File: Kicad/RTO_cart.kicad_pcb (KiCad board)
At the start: 2 copper layers, 68.1 x 90.1 mm, 22 parts, among them J1 2x22 card edge connector, J2 Oled 0.91" female, SW1 SW_Push, SW2 SW_Push, SW3 SW_Push, U1 74LVC245, U2 74LVC245, U3 74LVC245, U4 Teensy4.1, U5 74LVC245

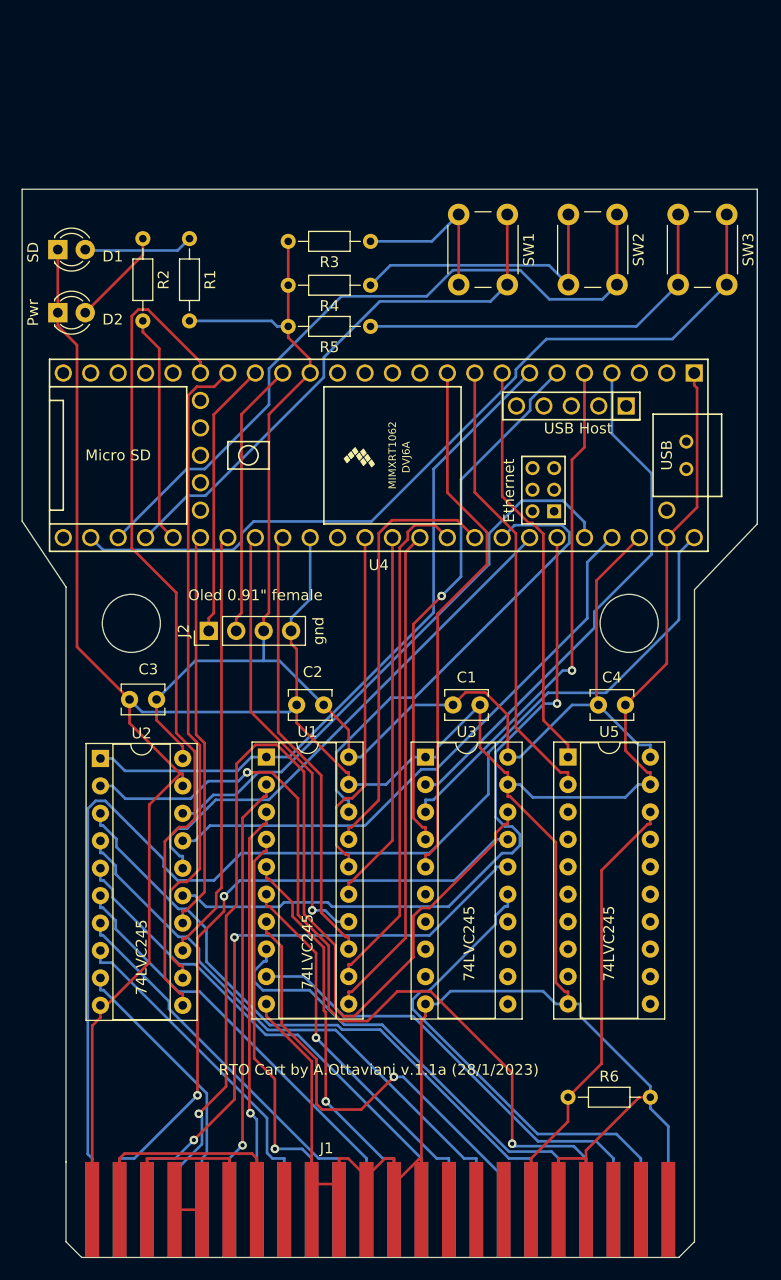
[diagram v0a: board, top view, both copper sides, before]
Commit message: Add files via upload
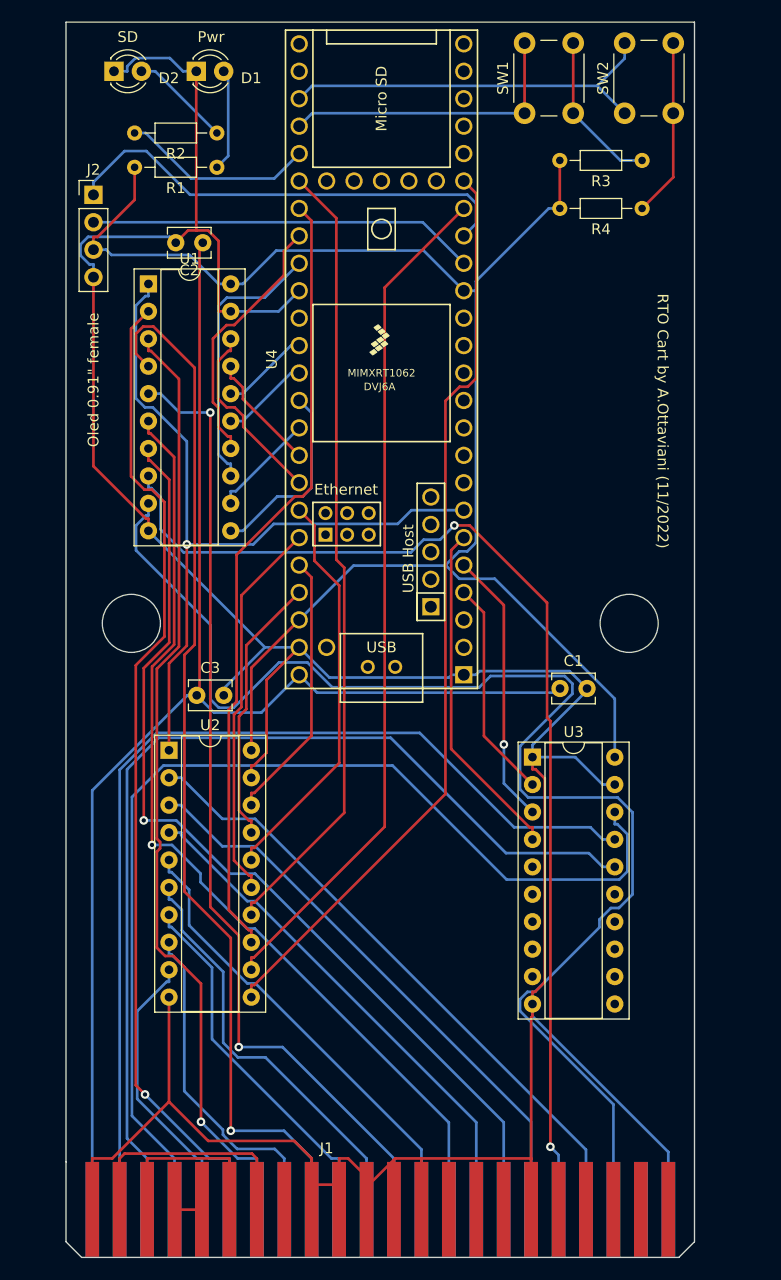
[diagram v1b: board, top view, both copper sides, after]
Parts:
- removed C4: 100nF, Capacitor_THT:C_Disc_D3.8mm_W2.6mm_P2.50mm
- removed R5: 1K, Resistor_THT:R_Axial_DIN0204_L3.6mm_D1.6mm_P7.62mm_Horizontal
- removed R6: 4K7, Resistor_THT:R_Axial_DIN0204_L3.6mm_D1.6mm_P7.62mm_Horizontal
- removed SW3: SW_Push, Button_Switch_THT:SW_PUSH_6mm
- removed U5: 74LVC245, Package_DIP:DIP-20_W7.62mm_Socket
- U1, U2, U3: value 74LVC245 -> 74LS245
- moved U1 45.2 mm to (96.5, 102.2)
- moved C2 44.2 mm to (101.6, 98.4)
- moved J2 41.8 mm to (91.4, 94.0), turned to 0 degrees
- moved R3 26.2 mm to (142.2, 90.8)
- moved R4 26.1 mm to (142.2, 95.2)
- moved D2 22.9 mm to (93.3, 82.5)
- moved D1 20.9 mm to (101.0, 82.5)
- moved R2 11.9 mm to (102.9, 88.3), turned to 180 degrees
- moved C1 10.0 mm to (134.6, 139.7)
- moved U3 9.91 mm to (132.1, 146.1)
- moved SW1 9.51 mm to (131.4, 86.4), turned to 90 degrees
- moved SW2 9.40 mm to (140.6, 86.4), turned to 90 degrees
- moved U4 8.89 mm to (118.1, 109.2), turned to 90 degrees
- moved R1 7.08 mm to (102.9, 91.4), turned to 180 degrees
- moved U2 6.40 mm to (98.4, 145.4)
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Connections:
- C1 pad 1: +3.3V -> +5V
- C2 pad 1: +3.3V -> +5V
- C3 pad 1: +3.3V -> +5V
- J1 pad 10: GND -> unconnected-(J1-Pad10)
- J1 pad 12: rst' -> GND
- J1 pad 3: ~{msync'} -> unconnected-(J1-Pad3)
- J1 pad 8: GND -> unconnected-(J1-Pad8)
- U3 pad 15: ~{msync'} -> unconnected-(U3-Pad15)
- U3 pad 5: ~{MSYNC} -> unconnected-(U3-Pad5)
- U4 pad 10: ~{MSYNC} -> unconnected-(U4-Pad10)
- U4 pad 26: BT3 -> unconnected-(U4-Pad26)
- U4 pad 8: DIR2 -> unconnected-(U4-Pad8)
- U4 pad 9: RST -> unconnected-(U4-Pad9)
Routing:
- net d7': track 43.9 -> 127.5 mm
- net BT3: track 76.9 -> 0.00 mm
- net d6': track 43.3 -> 102.9 mm, vias 0 -> 2
- net d2': track 38.6 -> 96.9 mm
- net d3': track 37.4 -> 89.7 mm, vias 1 -> 2
- net GND: track 368.8 -> 317.9 mm
- net d4': track 37.0 -> 87.9 mm
- net d1': track 37.9 -> 88.4 mm
- net d0': track 40.9 -> 91.3 mm
- net ~{MSYNC}: track 49.8 -> 0.00 mm
- net ~{msync'}: track 46.5 -> 0.00 mm
- net d5': track 44.6 -> 89.3 mm
- net RST: track 42.1 -> 0.00 mm
- net rst': track 41.5 -> 0.00 mm
- net DIR2: track 38.3 -> 0.00 mm
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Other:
- board size 68.1 x 90.1 mm -> 58.2 x 105.5 mm
- board text added: "RTO Cart by A.Ottaviani (11/2022)"
- board text removed: "RTO Cart by A.Ottaviani v.1.1a (28/1/2023)"
- board text removed: "gnd"

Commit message: Add files via upload
corrected the level shifter ICs to 74LVC245 instead of wrong typed 74LS245: WARNING! use only 74LVC245 chips, the other types could damage your Teensy becouse they output 5V instead of 3V3!
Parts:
- U1, U2, U3: value 74LS245 -> 74LVC245
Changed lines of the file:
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@@
       (effects (font (size 1 1) (thickness 0.15)))
     )
-    (fp_text value "74LS245" (at 3.81 25.19) (layer "F.Fab")
+    (fp_text value "74LVC245" (at 3.81 25.19) (layer "F.Fab")
       (effects (font (size 1 1) (thickness 0.15)))
     )
@@
       (effects (font (size 1 1) (thickness 0.15)))
     )
-    (fp_text value "74LS245" (at 3.81 25.19) (layer "F.Fab")
+    (fp_text value "74LVC245" (at 3.81 25.19) (layer "F.Fab")
       (effects (font (size 1 1) (thickness 0.15)))
     )
@@
       (effects (font (size 1 1) (thickness 0.15)))
     )
-    (fp_text value "74LS245" (at 3.81 25.19) (layer "F.Fab")
+    (fp_text value "74LVC245" (at 3.81 25.19) (layer "F.Fab")
       (effects (font (size 1 1) (thickness 0.15)))
     )

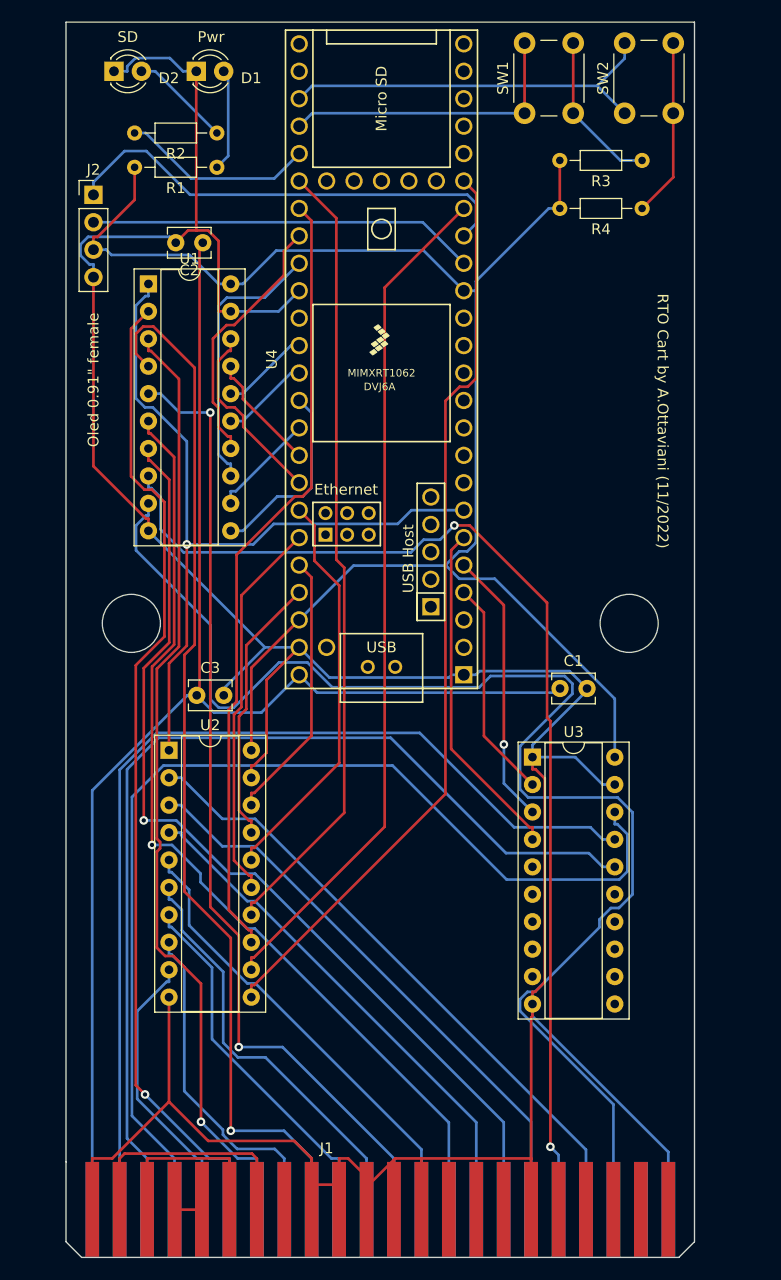
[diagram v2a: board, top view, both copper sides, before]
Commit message: Add files via upload
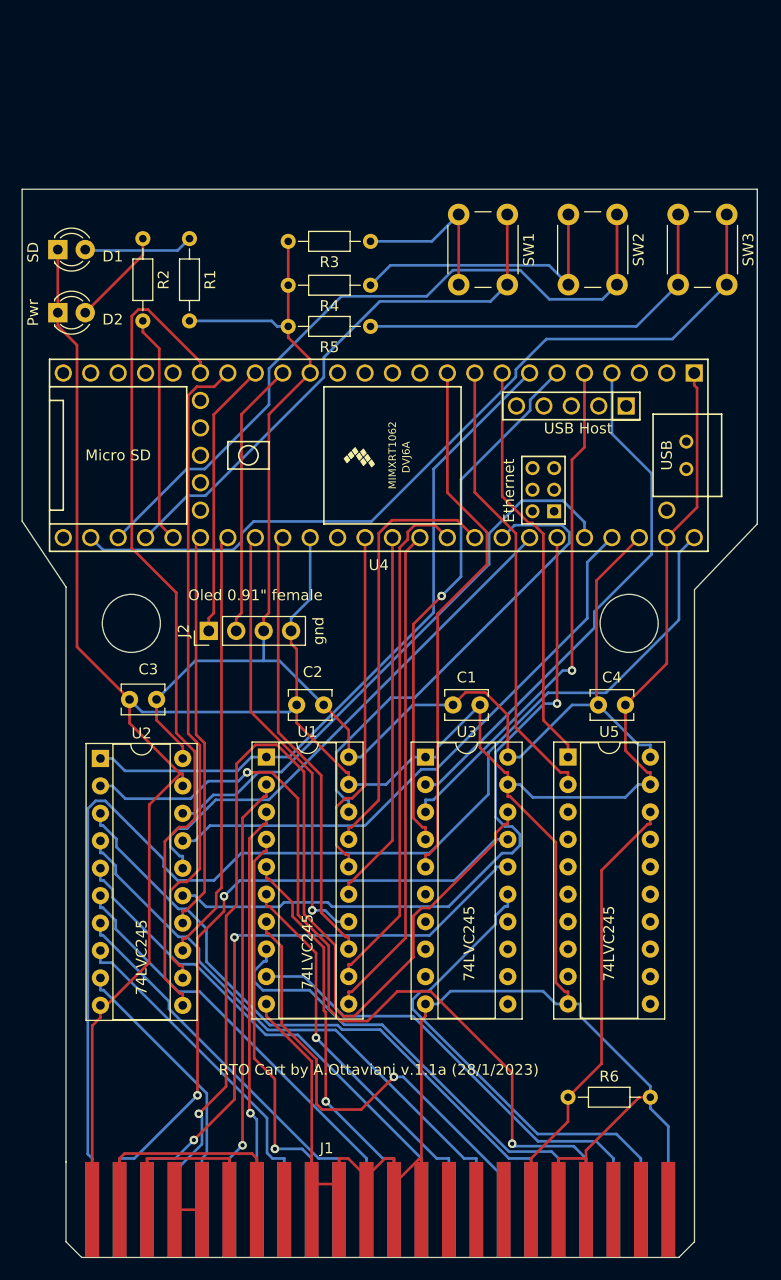
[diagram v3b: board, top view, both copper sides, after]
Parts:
- added C4: 100nF, Capacitor_THT:C_Disc_D3.8mm_W2.6mm_P2.50mm, F.Cu at (138.2, 141.2)
- added R5: 1K, Resistor_THT:R_Axial_DIN0204_L3.6mm_D1.6mm_P7.62mm_Horizontal, F.Cu at (117.1, 106.2)
- added R6: 4K7, Resistor_THT:R_Axial_DIN0204_L3.6mm_D1.6mm_P7.62mm_Horizontal, F.Cu at (135.4, 177.5)
- added SW3: SW_Push, Button_Switch_THT:SW_PUSH_6mm, F.Cu at (150.1, 95.8)
- added U5: 74LVC245, Package_DIP:DIP-20_W7.62mm_Socket, F.Cu at (135.4, 146.1)
- moved U1 45.2 mm to (107.5, 146.1)
- moved C2 44.2 mm to (112.8, 141.2)
- moved J2 41.8 mm to (102.1, 134.4), turned to 90 degrees
- moved R3 26.2 mm to (117.1, 98.3)
- moved R4 26.1 mm to (117.1, 102.4)
- moved D2 22.9 mm to (88.1, 104.9)
- moved D1 20.9 mm to (88.1, 99.1)
- moved R2 11.9 mm to (96.0, 98.0), turned to -90 degrees
- moved C1 10.0 mm to (124.7, 141.2)
- moved U3 9.91 mm to (122.2, 146.1)
- moved SW1 9.51 mm to (129.8, 95.8), turned to -90 degrees
- moved SW2 9.40 mm to (139.9, 95.8), turned to -90 degrees
- moved U4 8.89 mm to (117.9, 118.1), turned to 180 degrees
- moved R1 7.08 mm to (100.3, 98.0), turned to -90 degrees
- moved U2 6.40 mm to (92.1, 146.2)
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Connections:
- C1 pad 1: +5V -> +3.3V
- C2 pad 1: +5V -> +3.3V
- C3 pad 1: +5V -> +3.3V
- J1 pad 10: unconnected-(J1-Pad10) -> GND
- J1 pad 12: GND -> rst'
- J1 pad 3: unconnected-(J1-Pad3) -> ~{msync'}
- J1 pad 8: unconnected-(J1-Pad8) -> GND
- U3 pad 15: unconnected-(U3-Pad15) -> ~{msync'}
- U3 pad 5: unconnected-(U3-Pad5) -> ~{MSYNC}
- U4 pad 10: unconnected-(U4-Pad10) -> ~{MSYNC}
- U4 pad 26: unconnected-(U4-Pad26) -> BT3
- U4 pad 8: unconnected-(U4-Pad8) -> DIR2
- U4 pad 9: unconnected-(U4-Pad9) -> RST
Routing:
- net d7': track 127.5 -> 43.9 mm
- net BT3: track 0.00 -> 76.9 mm
- net d6': track 102.9 -> 43.3 mm, vias 2 -> 0
- net d2': track 96.9 -> 38.6 mm
- net d3': track 89.7 -> 37.4 mm, vias 2 -> 1
- net GND: track 317.9 -> 368.8 mm
- net d4': track 87.9 -> 37.0 mm
- net d1': track 88.4 -> 37.9 mm
- net d0': track 91.3 -> 40.9 mm
- net ~{MSYNC}: track 0.00 -> 49.8 mm
- net ~{msync'}: track 0.00 -> 46.5 mm
- net d5': track 89.3 -> 44.6 mm
- net RST: track 0.00 -> 42.1 mm
- net rst': track 0.00 -> 41.5 mm
- net DIR2: track 0.00 -> 38.3 mm
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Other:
- board size 58.2 x 105.5 mm -> 68.1 x 90.1 mm
- board text added: "RTO Cart by A.Ottaviani v.1.1a (28/1/2023)"
- board text added: "gnd"
- board text removed: "RTO Cart by A.Ottaviani (11/2022)"
